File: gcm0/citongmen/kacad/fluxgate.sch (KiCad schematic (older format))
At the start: 99 parts, among them J1 +12, J11 SWD, J2 ji_li, Q1 BC547, Q10 KIA50N03, Q11 BC547, Q12 BC557, Q13 BC557, Q14 BC547, Q15 BC557, Q16 BC547, Q17 BC547, Q18 BC547, Q19 BC547, Q2 BC557, Q3 BC547, Q4 BC557, Q5 BC547, Q6 BC557, Q7 KIA50N03, Q8 KIA50N03, Q9 KIA50N03, U1 LM7809_TO220, U2 LM2596S-5, U3 LM7805_TO220, U4 TL084, U5 STM32F030F4P6, U6 LM1117-3.3, U9 74HC595, Y1 8M

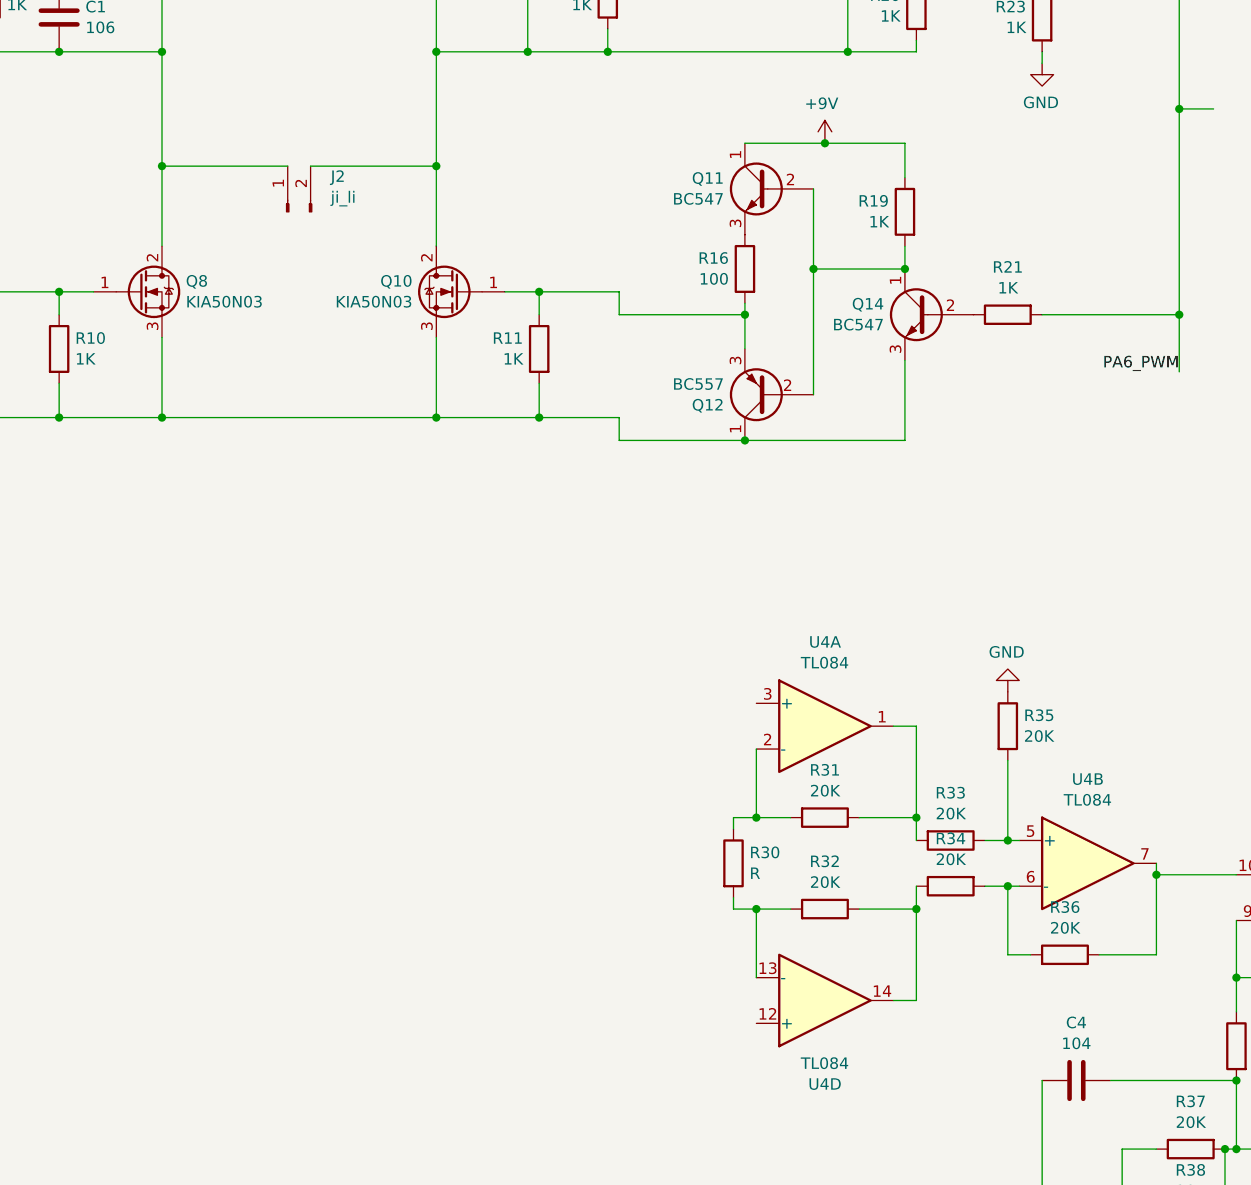
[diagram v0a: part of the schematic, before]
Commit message: 删掉无用文件
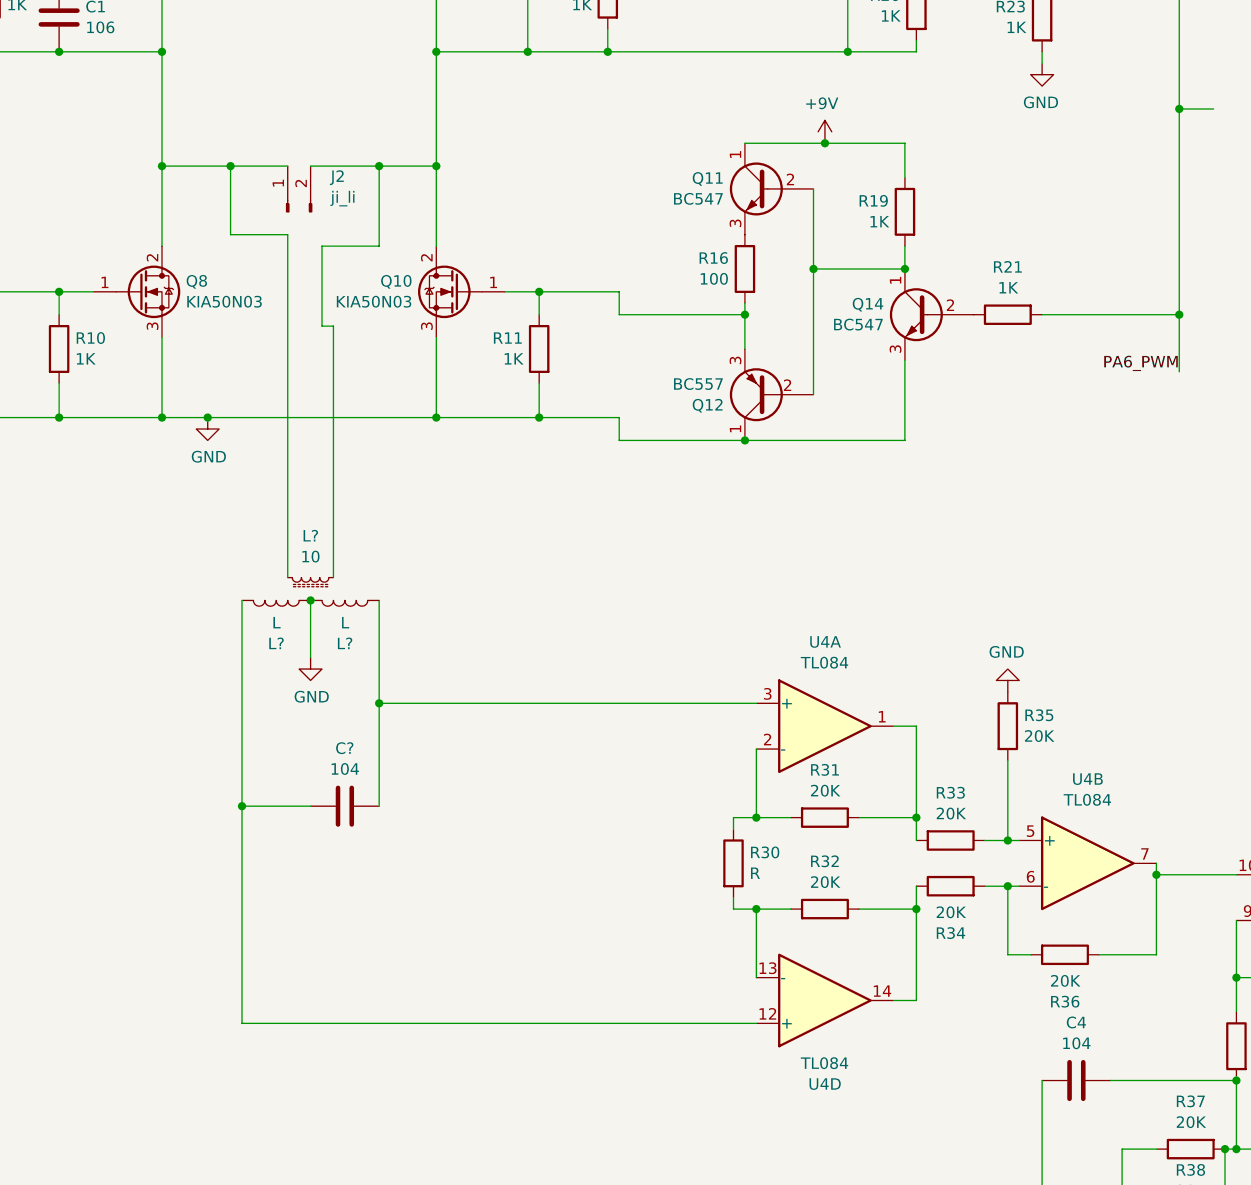
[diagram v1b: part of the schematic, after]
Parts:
- added C?: 104, symbol Device:C
- added L?: 10, symbol Device:L_Core_Ferrite_Small
- added L? (x2): L, symbol Device:L
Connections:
- net GND: now also Q10.3 (S), Q12.1 (C), Q14.3 (E), Q3.3 (E), Q6.1 (C), Q8.3 (S), R10.2, R11.2, L?.1, L?.2
- net at C1.2, J2.1 (Pin_1), Q4.1 (C)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: now also L?.2
- net at U4.3 (+): now also C?.1, L?.2
- net at U4.12 (+): now also C?.2, L?.1
- net at C3.2, J2.2 (Pin_2), Q10.2 (D)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: now also L?.1
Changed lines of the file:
@@
 Connection ~ 8000 1300
 Wire Wire Line
-	4700 4100 5900 4100
+	4700 4100 4900 4100
 Connection ~ 4700 4100
 Connection ~ 5900 4100
@@
 	4700 2500 4700 3000
 Wire Wire Line
-	5250 3000 4700 3000
+	5250 3000 5000 3000
 Connection ~ 4700 3000
 Wire Wire Line
 	4700 3000 4700 3350
 Wire Wire Line
-	5350 3000 5900 3000
+	5350 3000 5650 3000
 Connection ~ 5900 3000
 Wire Wire Line
@@
 F 3 "~" H 8150 6150 50  0001 C CNN
 	1    8150 6150
-	0    -1   1    0
+	0    -1   -1   0
 $EndComp
 $Comp
@@
 F 3 "~" H 8650 6450 50  0001 C CNN
 	1    8650 6450
-	0    1    -1   0
+	0    1    1    0
 $EndComp
 Wire Wire Line
@@
 	9950 7300 10300 7300
 Connection ~ 9950 7300
+$Comp
+L Device:L_Core_Ferrite_Small L?
+U 1 1 60E8B5A8
+P 5350 4800
+F 0 "L?" V 5169 4800 50  0000 C CNN
+F 1 "10" V 5260 4800 50  0000 C CNN
+F 2 "" H 5350 4800 50  0001 C CNN
+F 3 "~" H 5350 4800 50  0001 C CNN
+	1    5350 4800
+	0    1    1    0
+$EndComp
+Wire Wire Line
+	5250 4800 5250 3300
+Wire Wire Line
+	5250 3300 5000 3300
+Wire Wire Line
+	5000 3300 5000 3000
+Connection ~ 5000 3000
+Wire Wire Line
+	5000 3000 4700 3000
+Wire Wire Line
+	5450 4800 5450 3700
+Wire Wire Line
+	5450 3700 5400 3700
+Wire Wire Line
+	5400 3700 5400 3350
+Wire Wire Line
+	5400 3350 5650 3350
+Wire Wire Line
+	5650 3350 5650 3000
+Connection ~ 5650 3000
+Wire Wire Line
+	5650 3000 5900 3000
+$Comp
+L Device:L L?
+U 1 1 60ECEB72
+P 5200 4900
+F 0 "L?" V 5390 4900 50  0000 C CNN
+F 1 "L" V 5299 4900 50  0000 C CNN
+F 2 "" H 5200 4900 50  0001 C CNN
+F 3 "~" H 5200 4900 50  0001 C CNN
+	1    5200 4900
+	0    -1   1    0
+$EndComp
+$Comp
+L Device:L L?
+U 1 1 60ED0F8B
+P 5500 4900
+F 0 "L?" V 5690 4900 50  0000 C CNN
+F 1 "L" V 5599 4900 50  0000 C CNN
+F 2 "" H 5500 4900 50  0001 C CNN
+F 3 "~" H 5500 4900 50  0001 C CNN
+	1    5500 4900
+	0    -1   1    0
+$EndComp
+Wire Wire Line
+	5350 4900 5350 5150
+Connection ~ 5350 4900
+$Comp
+L power:GND #PWR?
+U 1 1 60F5890A
+P 5350 5150
+F 0 "#PWR?" H 5350 4900 50  0001 C CNN
+F 1 "GND" H 5355 4977 50  0000 C CNN
+F 2 "" H 5350 5150 50  0001 C CNN
+F 3 "" H 5350 5150 50  0001 C CNN
+	1    5350 5150
+	1    0    0    -1
+$EndComp
+Wire Wire Line
+	5650 4900 5650 5350
+Wire Wire Line
+	5650 5350 7300 5350
+Wire Wire Line
+	5050 4900 5050 5800
+Wire Wire Line
+	5050 6750 7300 6750
+$Comp
+L Device:C C?
+U 1 1 60E8E98A
+P 5500 5800
+F 0 "C?" V 5248 5800 50  0000 C CNN
+F 1 "104" V 5339 5800 50  0000 C CNN
+F 2 "" H 5538 5650 50  0001 C CNN
+F 3 "~" H 5500 5800 50  0001 C CNN
+	1    5500 5800
+	0    1    1    0
+$EndComp
+Wire Wire Line
+	5650 5800 5650 5350
+Connection ~ 5650 5350
+Wire Wire Line
+	5350 5800 5050 5800
+Connection ~ 5050 5800
+Wire Wire Line
+	5050 5800 5050 6750
+$Comp
+L power:GND #PWR?
+U 1 1 60E90175
+P 4900 4100
+F 0 "#PWR?" H 4900 3850 50  0001 C CNN
+F 1 "GND" H 4905 3927 50  0000 C CNN
+F 2 "" H 4900 4100 50  0001 C CNN
+F 3 "" H 4900 4100 50  0001 C CNN
+	1    4900 4100
+	1    0    0    -1
+$EndComp
+Connection ~ 4900 4100
+Wire Wire Line
+	4900 4100 5900 4100
 $EndSCHEMATC
